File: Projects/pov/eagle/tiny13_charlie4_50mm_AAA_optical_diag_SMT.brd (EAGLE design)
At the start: 49.8 x 49.8 mm, 25 parts, among them IC1 TINY13-20SU, X1 USBPCB

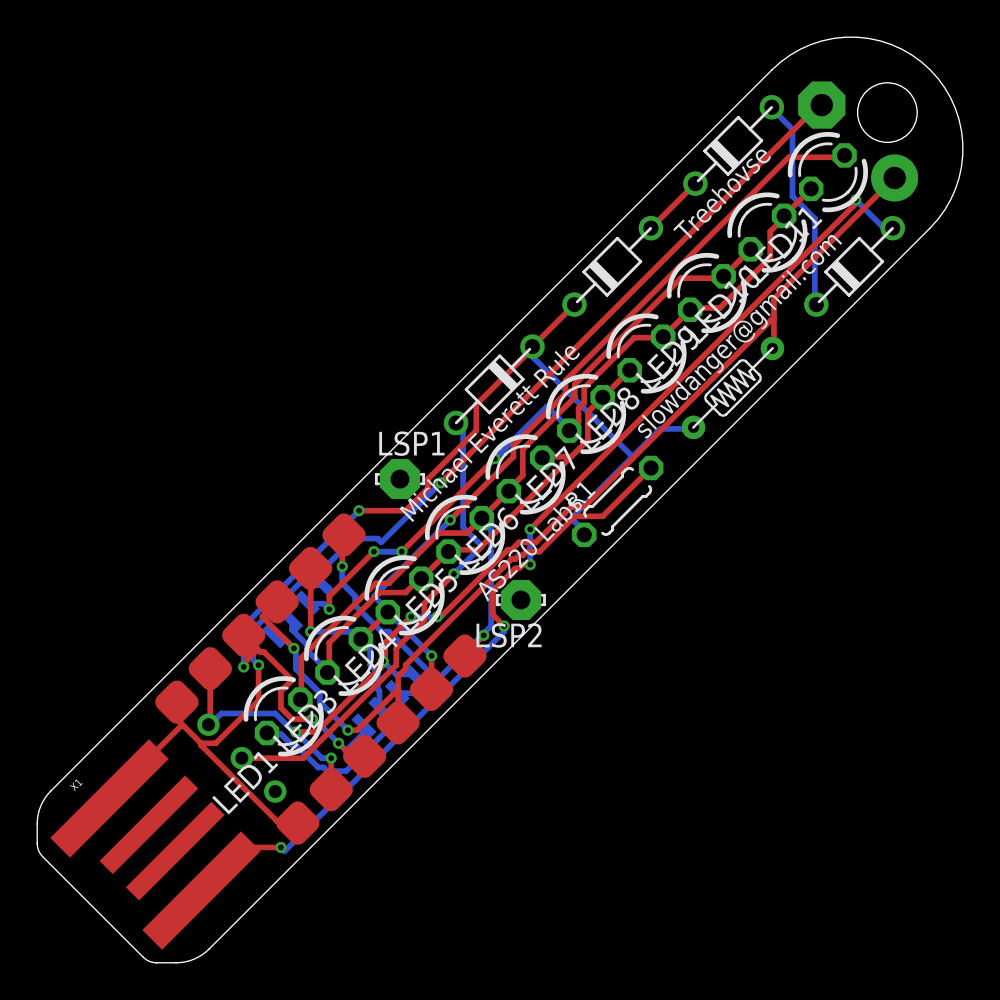
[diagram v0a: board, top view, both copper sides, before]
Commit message: update contact information
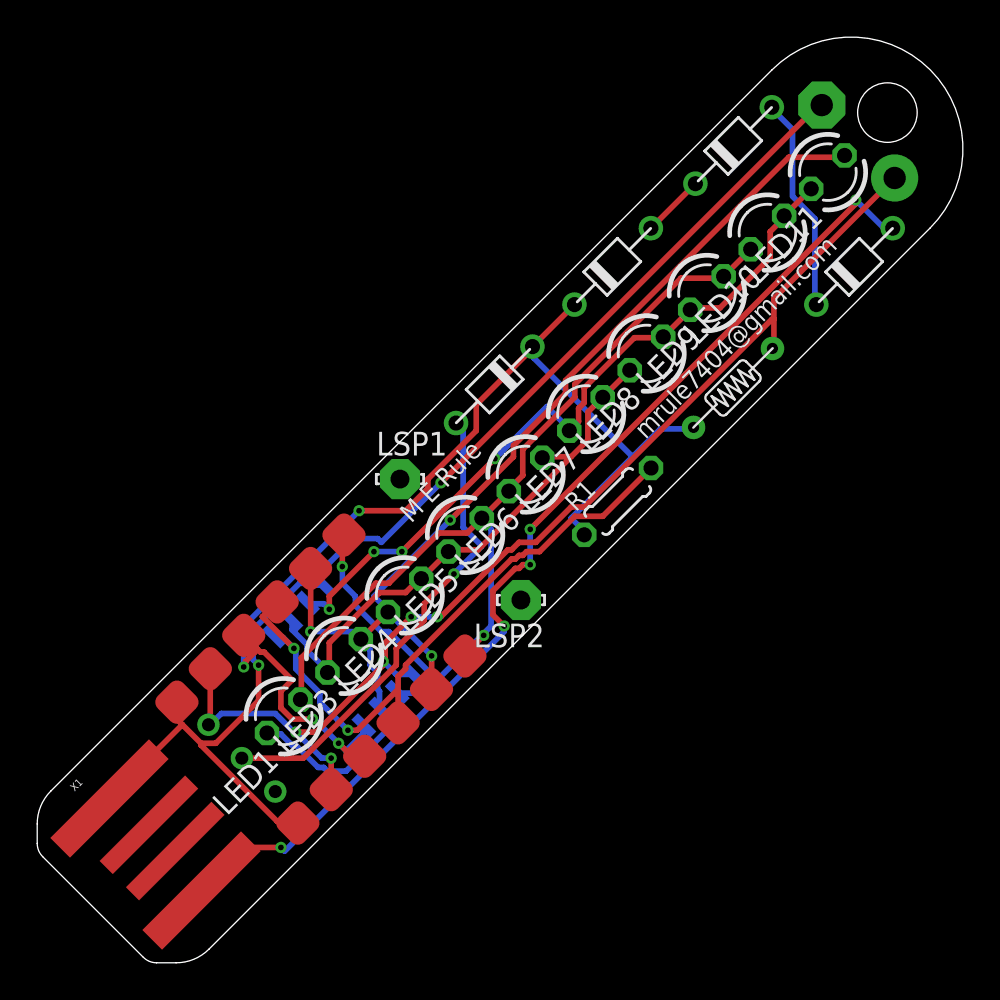
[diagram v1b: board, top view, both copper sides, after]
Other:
- board text added: "M E Rule"
- board text added: "mrule7404@gmail.com"
- board text removed: "AS220 Labs"
- board text removed: "Michael Everett Rule"
- board text removed: "Treehovse"
- board text removed: "slowdanger@gmail.com"
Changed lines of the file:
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@@
 <hole x="45.7" y="45.7" drill="3.2"/>
 <wire x1="39.5" y1="48" x2="48" y2="39.5" width="0" layer="20" curve="-180"/>
-<text x="20.1" y="23.6" size="1.016" layer="21" font="vector" ratio="15" rot="R45">Michael Everett Rule</text>
-<text x="34.9" y="38.7" size="1.016" layer="21" font="vector" ratio="15" rot="R45">Treehovse</text>
-<text x="24.2" y="19.4" size="1.016" layer="21" font="vector" ratio="15" rot="R45">AS220 Labs</text>
-<text x="32.7" y="28.1" size="1.016" layer="21" font="vector" ratio="15" rot="R45">slowdanger@gmail.com</text>
+<text x="20.1" y="23.6" size="1.016" layer="21" font="vector" ratio="15" rot="R45">M E Rule</text>
+<text x="32.7" y="28.1" size="1.016" layer="21" font="vector" ratio="15" rot="R45">mrule7404@gmail.com</text>
 </plain>
 <attributes>
